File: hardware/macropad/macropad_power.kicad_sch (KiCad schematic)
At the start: 27 parts, among them J6 Conn_01x03_Socket, J8 Conn_01x02, Q1 Q_PMOS, Q2 FS8205A, SW10 SW_SPDT, U6 TP4056-42-ESOP8, U7 DW01A, U8 RT8010AGQW, U9 LP2992IM5-3.3/NOPB

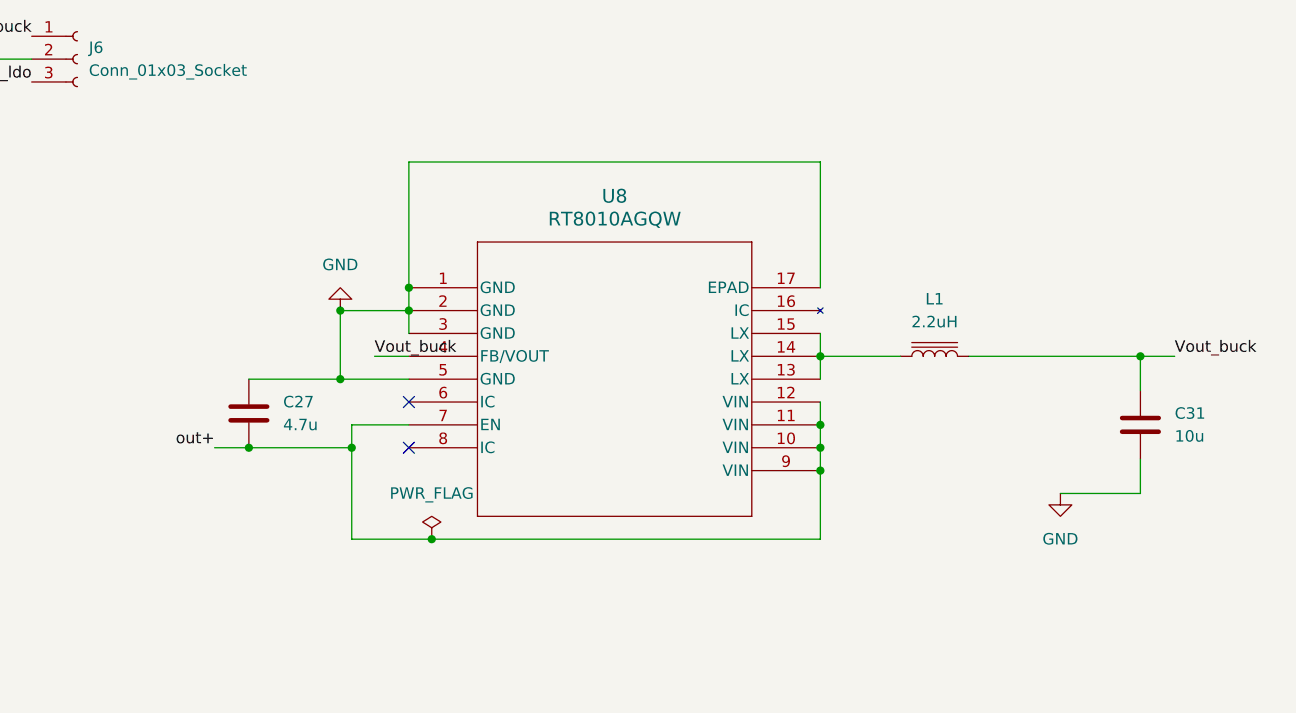
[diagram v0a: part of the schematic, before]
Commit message: routing phase 2
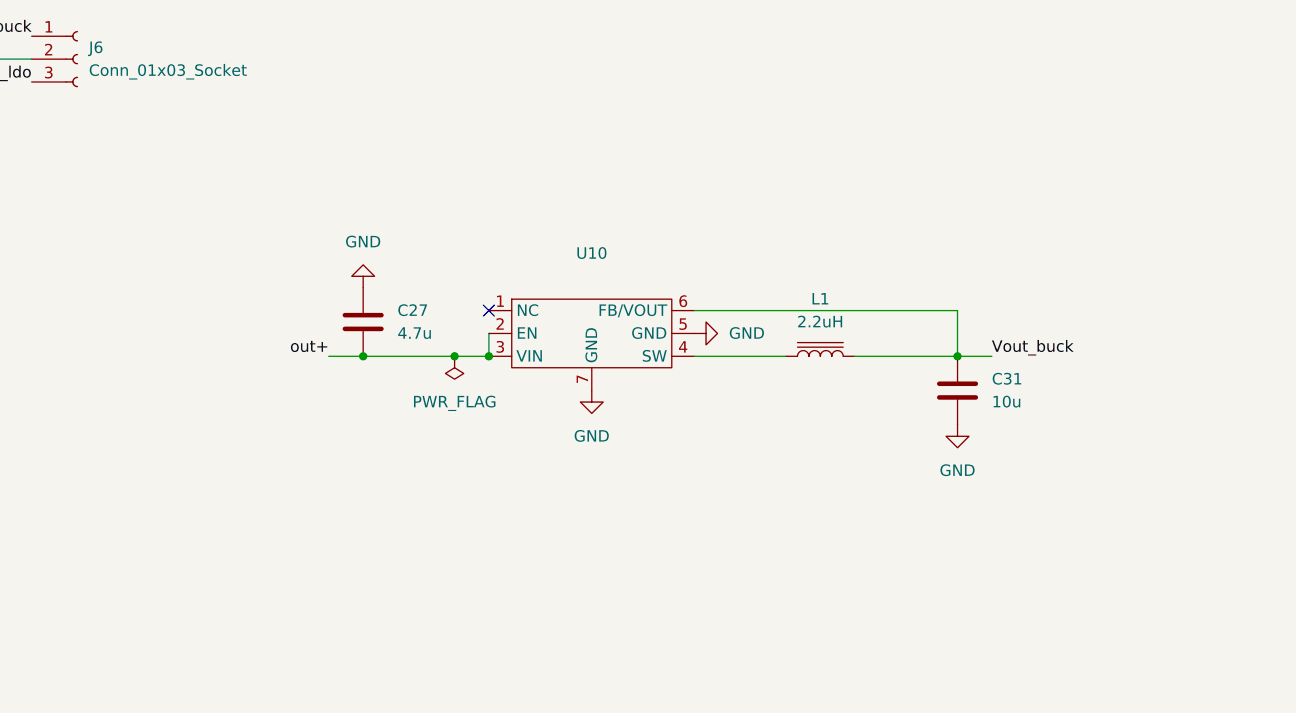
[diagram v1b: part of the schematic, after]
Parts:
- removed U8: RT8010AGQW, RT8010:WQFN16_RT8010_RIT, symbol RT8010:RT8010AGQW
- added U10: ~, RT8010:WDFN-6L, symbol rt8010:rt8010_wdfn
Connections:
- net GND: now also U10.5 (GND), U10.7 (GND)
- net Vout_buck: now also U10.6 (FB/VOUT)
- net out+: now also U10.2 (EN), U10.3 (VIN)
- net at L1.1: now also U10.4 (SW)
- no-connect marks 4 -> 3
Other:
- moved on the sheet: C27, C31, L1
